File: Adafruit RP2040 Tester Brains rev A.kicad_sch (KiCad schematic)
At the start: 47 parts, among them IC1 WS2811-SOP8, Q1 DMG34x5, Q2 DMG34x5, Q3 BSS138, Q4 BSS138, Q5 BSS138, SW1 12mm SMT, SW2 DPDT SLIDE, X1 USB A, X2 MicroSD, X3 TESTER_PROGCABLE_FLIP

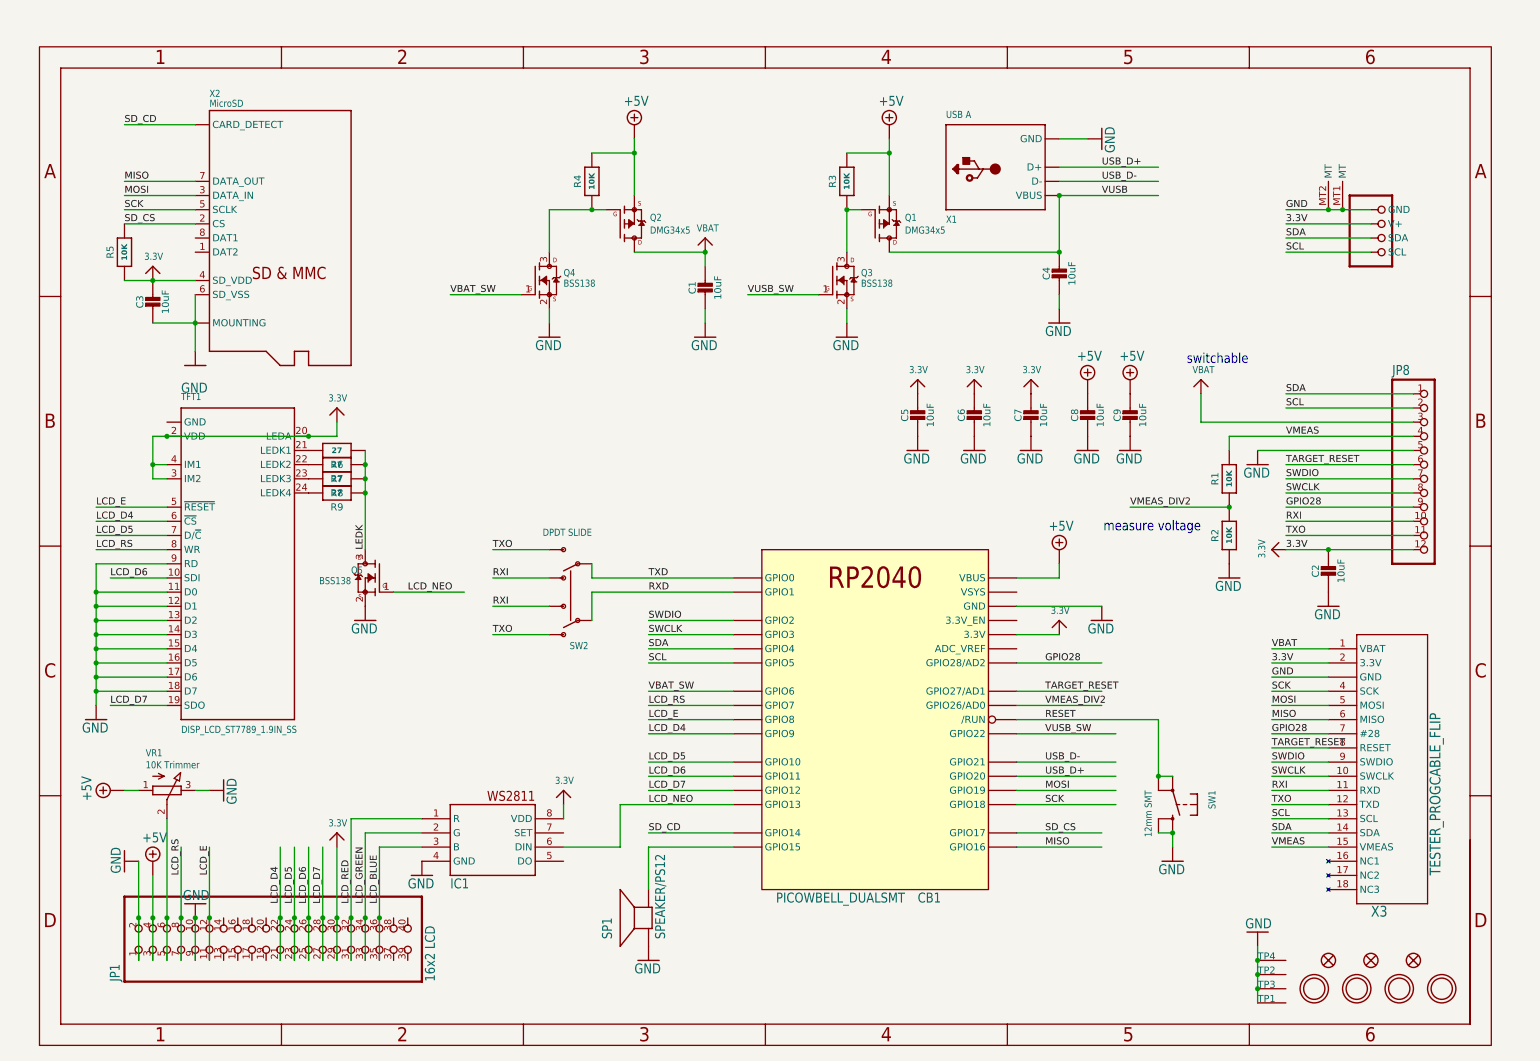
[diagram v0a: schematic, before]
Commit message: More migration to kKiCAD
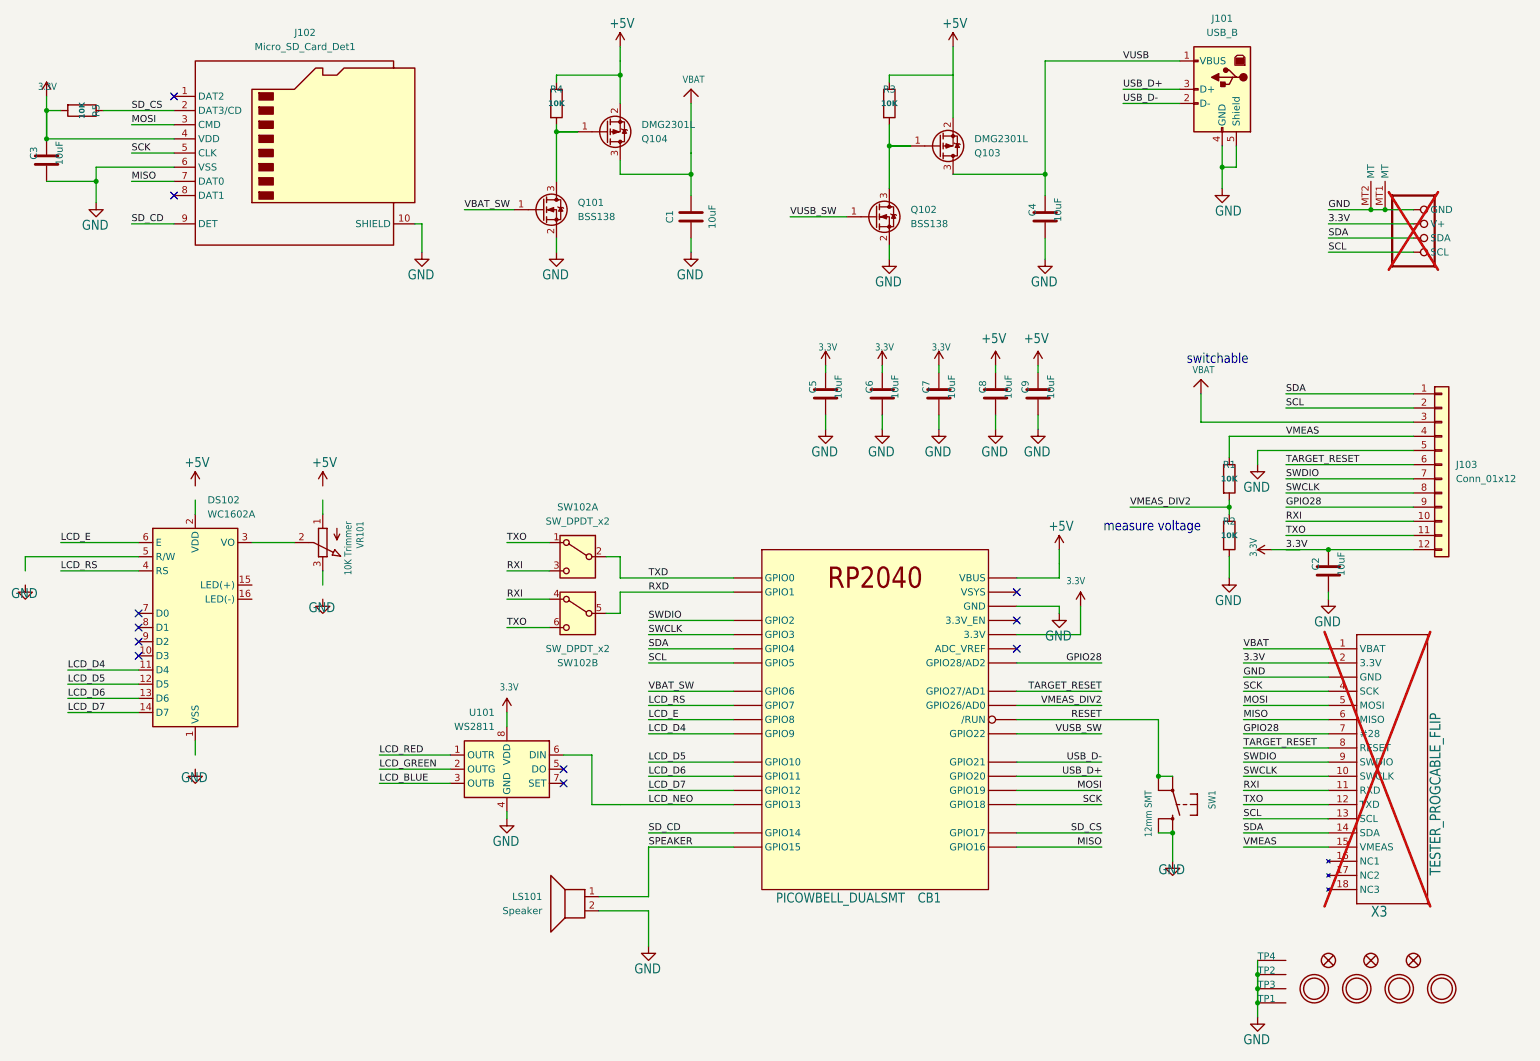
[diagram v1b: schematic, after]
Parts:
- removed IC1: WS2811-SOP8, Adafruit RP2040 Tester Brains rev A:SO08-SKINNYPADS, symbol Adafruit RP2040 Tester Brains rev A-eagle-import:WS2811-SOP8
- removed JP1: 16x2 LCD, Adafruit RP2040 Tester Brains rev A:2X20_SMT_MALE, symbol Adafruit RP2040 Tester Brains rev A-eagle-import:PINHD-2X20_SMT
- removed JP8: HEADER-1X12OVAL, Adafruit RP2040 Tester Brains rev A:1X12_OVAL, symbol Adafruit RP2040 Tester Brains rev A-eagle-import:HEADER-1X12OVAL
- removed Q1, Q2: DMG34x5, Adafruit RP2040 Tester Brains rev A:SOT23-WIDE, symbol Adafruit RP2040 Tester Brains rev A-eagle-import:MOSFET-PWIDE
- removed Q3, Q4, Q5: BSS138, Adafruit RP2040 Tester Brains rev A:SOT23-WIDE, symbol Adafruit RP2040 Tester Brains rev A-eagle-import:MOSFET-NWIDE
- removed R6, R7, R8, R9: 27, Adafruit RP2040 Tester Brains rev A:0603-NO, symbol Adafruit RP2040 Tester Brains rev A-eagle-import:RESISTOR_0603_NOOUT
- removed SP1: SPEAKER/PS12, Adafruit RP2040 Tester Brains rev A:PS12, symbol Adafruit RP2040 Tester Brains rev A-eagle-import:SPEAKER/PS12
- removed SW2: DPDT SLIDE, Adafruit RP2040 Tester Brains rev A:EG1390, symbol Adafruit RP2040 Tester Brains rev A-eagle-import:SWITCH_DPDTEG1390
- removed TFT1: DISP_LCD_ST7789_1.9IN_SS, Adafruit RP2040 Tester Brains rev A:TFT_1.9IN_170X320_30P_SS, symbol Adafruit RP2040 Tester Brains rev A-eagle-import:DISP_LCD_ST7789_1.9IN_SS
- removed VR1: 10K Trimmer, Adafruit RP2040 Tester Brains rev A:TRIMPOT_BOURNS_TC33X-2, symbol Adafruit RP2040 Tester Brains rev A-eagle-import:TRIMPOTTC33X-2
- removed X1: USB A, Adafruit RP2040 Tester Brains rev A:USB_HOST-SMT, symbol Adafruit RP2040 Tester Brains rev A-eagle-import:USB_TYPEA_SMT
- removed X2: MicroSD, Adafruit RP2040 Tester Brains rev A:MICROSD, symbol Adafruit RP2040 Tester Brains rev A-eagle-import:MICROSD
- added DS102: WC1602A, Display:WC1602A, symbol Display_Character:WC1602A
- added J101: USB_B, Connector_USB:USB_A_Molex_67643_Horizontal, symbol Connector:USB_B
- added J102: Micro_SD_Card_Det1, Connector_Card:microSD_HC_Molex_104031-0811, symbol Connector:Micro_SD_Card_Det1
- added J103: Conn_01x12, Connector_PinSocket_2.54mm:PinSocket_1x12_P2.54mm_Horizontal, symbol Connector_Generic:Conn_01x12
- added LS101: Speaker, Buzzer_Beeper:Buzzer_12x9.5RM7.6, symbol Device:Speaker
- added Q101, Q102: BSS138, Package_TO_SOT_SMD:SOT-23, symbol Transistor_FET:BSS138
- added Q103, Q104: DMG2301L, Package_TO_SOT_SMD:SOT-23, symbol Transistor_FET:DMG2301L
- added SW102: SW_DPDT_x2, Button_Switch_THT:SW_CK_JS202011AQN_DPDT_Angled, symbol Switch:SW_DPDT_x2
- added U101: WS2811, Package_SO:SOIC-8_3.9x4.9mm_P1.27mm, symbol Driver_LED:WS2811
- added VR101: 10K Trimmer, Adafruit RP2040 Tester Brains rev A:TRIMPOT_BOURNS_TC33X-2, symbol Adafruit RP2040 Tester Brains rev A-eagle-import:TRIMPOTTC33X-2
- C1, C2, C3, C4, C5, C6, C7, C8, C9: footprint Adafruit RP2040 Tester Brains rev A:0805-NO -> Capacitor_SMD:C_0805_2012Metric_Pad1.18x1.45mm_HandSolder; symbol Adafruit RP2040 Tester Brains rev A-eagle-import:CAP_CERAMIC0805-NOOUTLINE -> Device:C
- CONN1, X3: now not fitted; now left out of the parts list
- FID1, FID2, FID3: footprint Adafruit RP2040 Tester Brains rev A:FIDUCIAL_1MM -> Fiducial:Fiducial_1mm_Mask3mm
- R1, R2, R3, R4, R5: footprint Adafruit RP2040 Tester Brains rev A:0603-NO -> Resistor_SMD:R_0603_1608Metric_Pad0.98x0.95mm_HandSolder; symbol Adafruit RP2040 Tester Brains rev A-eagle-import:RESISTOR_0603_NOOUT -> Device:R
- U$10, U$7, U$8, U$9: footprint Adafruit RP2040 Tester Brains rev A:MOUNTINGHOLE_3.0_PLATEDTHIN -> MountingHole:MountingHole_3.2mm_M3; symbol Adafruit RP2040 Tester Brains rev A-eagle-import:MOUNTINGHOLE3.0THIN -> Adafruit RP2040 Tester Brains rev A-eagle-import:adafruit_electromech_MOUNTINGHOLE3.0THIN
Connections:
- net +5V: now also R4.1, Q103.2 (S), Q104.2 (S); no longer R3.2, R4.2
- net 3.3V: now also R5.2, J102.4 (VDD), J103.12 (Pin_12), U101.8 (VDD); no longer R5.1
- net GND: now also R2.2, J101.4 (GND), J101.5 (Shield), J102.10 (SHIELD), J102.6 (VSS), J103.5 (Pin_5), LS101.2, Q101.2 (S), Q102.2 (S), U101.4 (GND); no longer R2.1
- net GPIO28: now also J103.9 (Pin_9)
- net LCD_BLUE: now also U101.3 (OUTB)
- net LCD_D4: now also DS102.11 (D4)
- net LCD_D5: now also DS102.12 (D5)
- net LCD_D6: now also DS102.13 (D6)
- net LCD_D7: now also DS102.14 (D7)
- net LCD_E: now also DS102.6 (E)
- net LCD_GREEN: now also U101.2 (OUTG)
- net LCD_NEO: now also U101.6 (DIN)
- net LCD_RED: now also U101.1 (OUTR)
- net LCD_RS: now also DS102.4 (RS)
- net MISO: now also J102.7 (DAT0)
- net MOSI: now also J102.3 (CMD)
- net RXD: now also SW102.5 (B)
- net RXI: now also J103.10 (Pin_10), SW102.3 (C), SW102.4 (A)
- net SCK: now also J102.5 (CLK)
- net SCL: now also J103.2 (Pin_2)
- net SDA: now also J103.1 (Pin_1)
- net SD_CD: now also J102.9 (DET)
- net SD_CS: now also R5.1, J102.2 (DAT3/CD); no longer R5.2
- net SWCLK: now also J103.8 (Pin_8)
- net SWDIO: now also J103.7 (Pin_7)
- net TARGET_RESET: now also J103.6 (Pin_6)
- net TXD: now also SW102.2 (B)
- net TXO: now also J103.11 (Pin_11), SW102.1 (A), SW102.6 (C)
- net USB_D+: now also J101.3 (D+)
- net USB_D-: now also J101.2 (D-)
- net VBAT: now also J103.3 (Pin_3), Q104.3 (D)
- net VBAT_SW: now also Q101.1 (G)
- net VMEAS: now also R1.1, J103.4 (Pin_4); no longer R1.2
- net VMEAS_DIV2: now also R1.2, R2.1; no longer R1.1, R2.2
- net VUSB: now also J101.1 (VBUS), Q103.3 (D)
- net VUSB_SW: now also Q102.1 (G)
- net SPEAKER: now reaches CB1.S39 (GPIO15), CB1.S40 (GPIO15)
- net SPEAKER: now also LS101.1
- new net: Q101.3 (D), Q104.1 (G), R4.2
- new net: Q102.3 (D), Q103.1 (G), R3.2
- new net: DS102.3 (VO), VR101.2 (S)
- no-connect marks 0 -> 11
